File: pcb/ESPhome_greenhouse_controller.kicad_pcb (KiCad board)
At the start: 2 copper layers, 15 parts, among them K1 SANYOU_SRD_Form_C, K2 SANYOU_SRD_Form_C, K3 SANYOU_SRD_Form_C, K4 SANYOU_SRD_Form_C, K5 SANYOU_SRD_Form_C, K6 SANYOU_SRD_Form_C, U1 PC817, U2 PC817, U3 INA219AxD, U4 INA219AxD

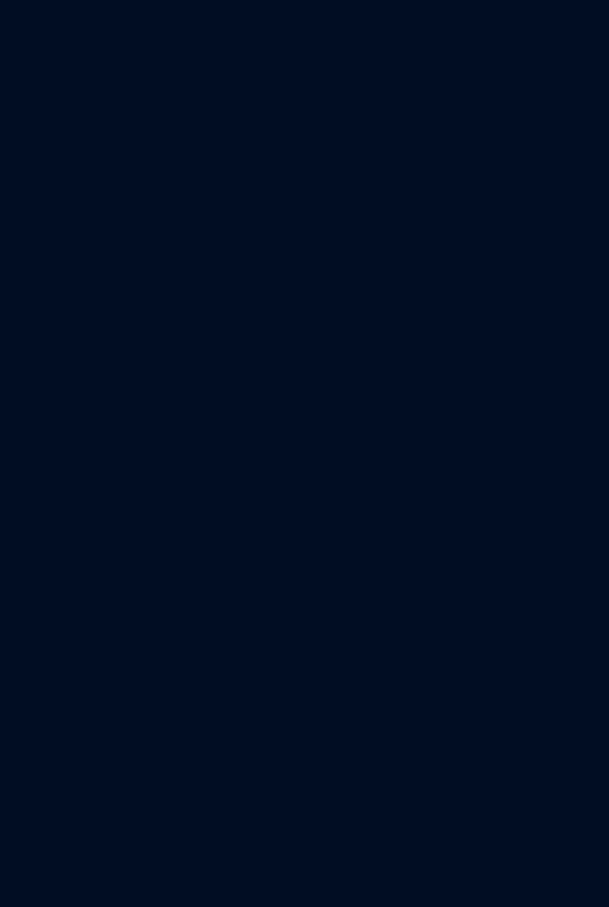
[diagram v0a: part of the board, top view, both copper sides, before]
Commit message: update
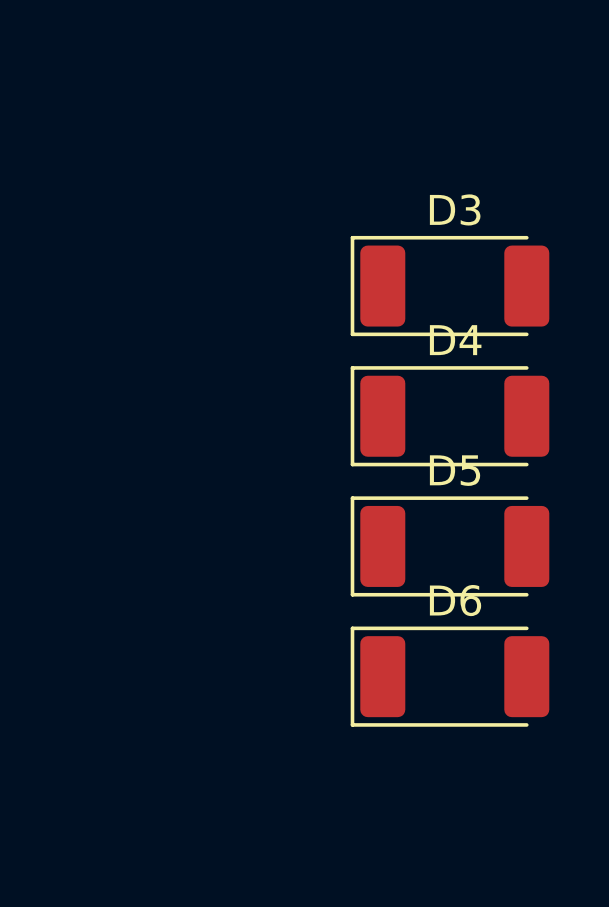
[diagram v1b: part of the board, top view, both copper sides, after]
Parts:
- added D3: SM4007, Diode_SMD:D_MELF, F.Cu at (190.5, 48.4)
- added D4: SM4007, Diode_SMD:D_MELF, F.Cu at (190.5, 52.7)
- added D5: SM4007, Diode_SMD:D_MELF, F.Cu at (190.5, 57.1)
- added D6: SM4007, Diode_SMD:D_MELF, F.Cu at (190.5, 61.4)
- U1, U2: value PC817 -> EL817

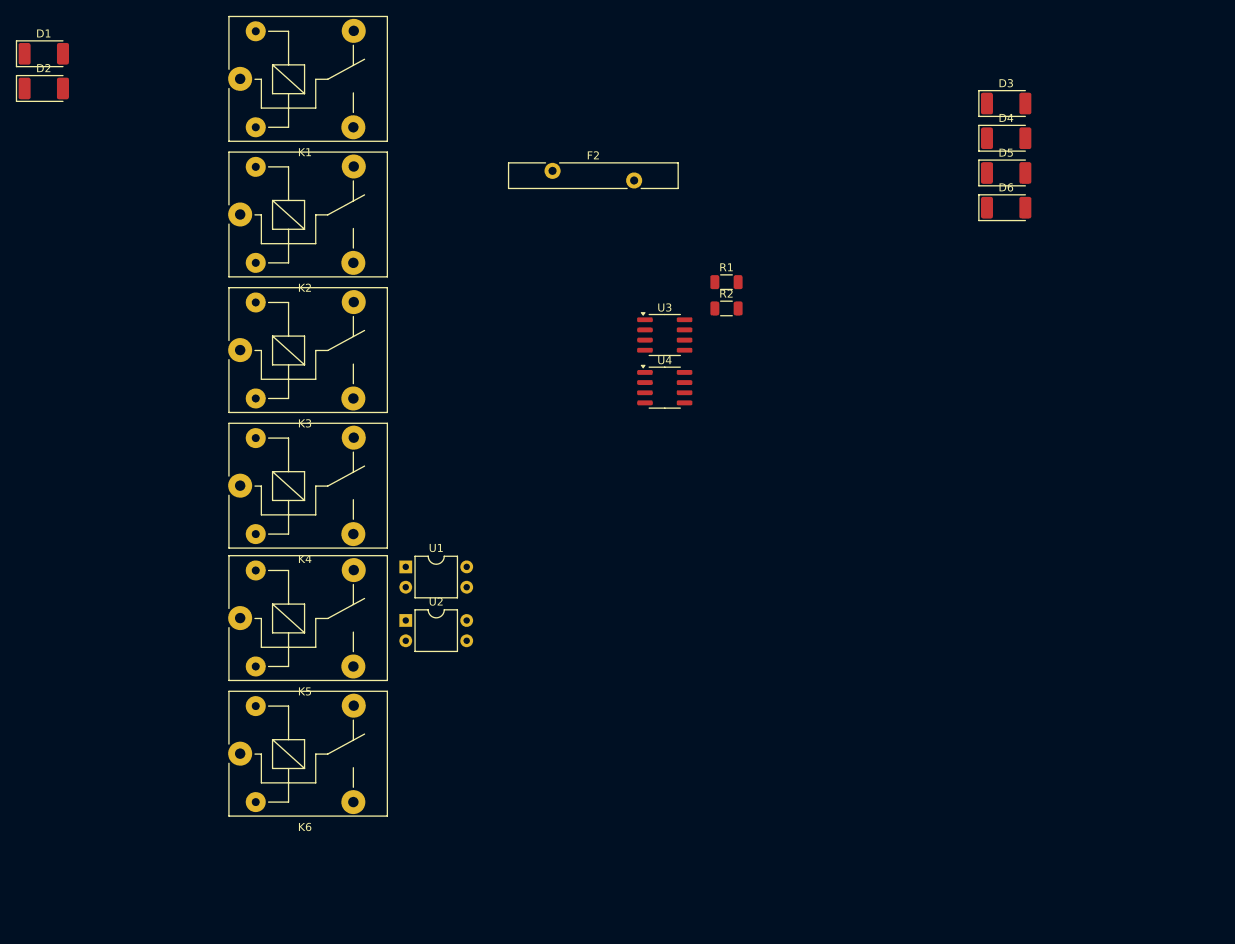
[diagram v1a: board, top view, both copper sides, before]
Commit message: update
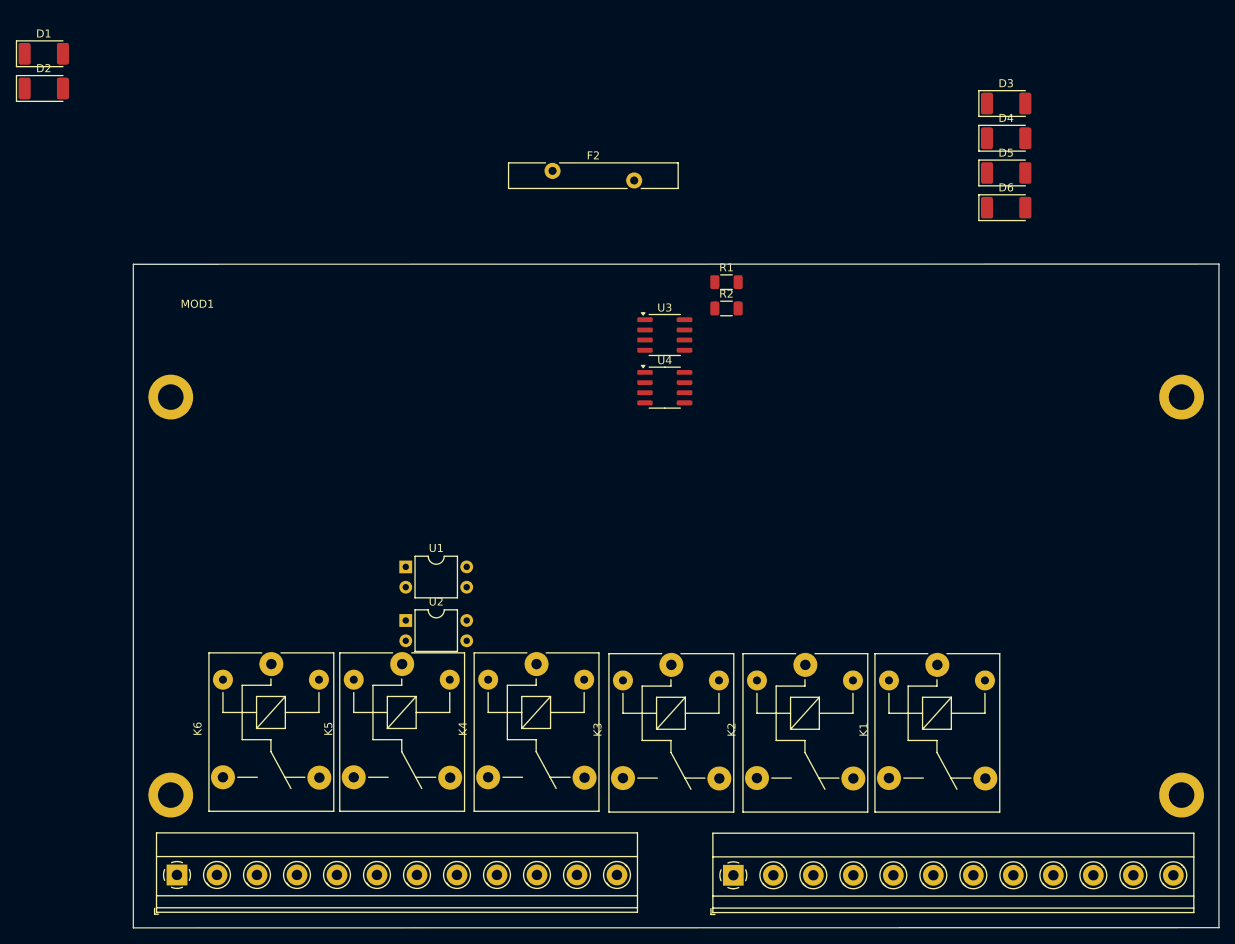
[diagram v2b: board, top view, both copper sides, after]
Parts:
- added MOD1: ~, kadex:ZD1008, F.Cu at (81.4, 110.0)
- moved K1 113.8 mm to (181.9, 118.5), turned to -90 degrees
- moved K2 90.3 mm to (165.4, 118.5), turned to -90 degrees
- moved K3 66.7 mm to (148.7, 118.5), turned to -90 degrees
- moved K4 43.2 mm to (131.8, 118.5), turned to -90 degrees
- moved K5 21.1 mm to (115.0, 118.5), turned to -90 degrees
- moved K6 11.9 mm to (98.7, 118.5), turned to -90 degrees
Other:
- board outline added: 135.7 x 83 mm
